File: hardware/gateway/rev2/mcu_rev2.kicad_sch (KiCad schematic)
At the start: 35 parts, among them IC1 STM8L151K4T6, IC5 MB85RC64TAPNF-G-BDERE1, J1 G8250041000YEU, J2 M20-9770342, Q1 IRLML6402TRPBF, U1 2462

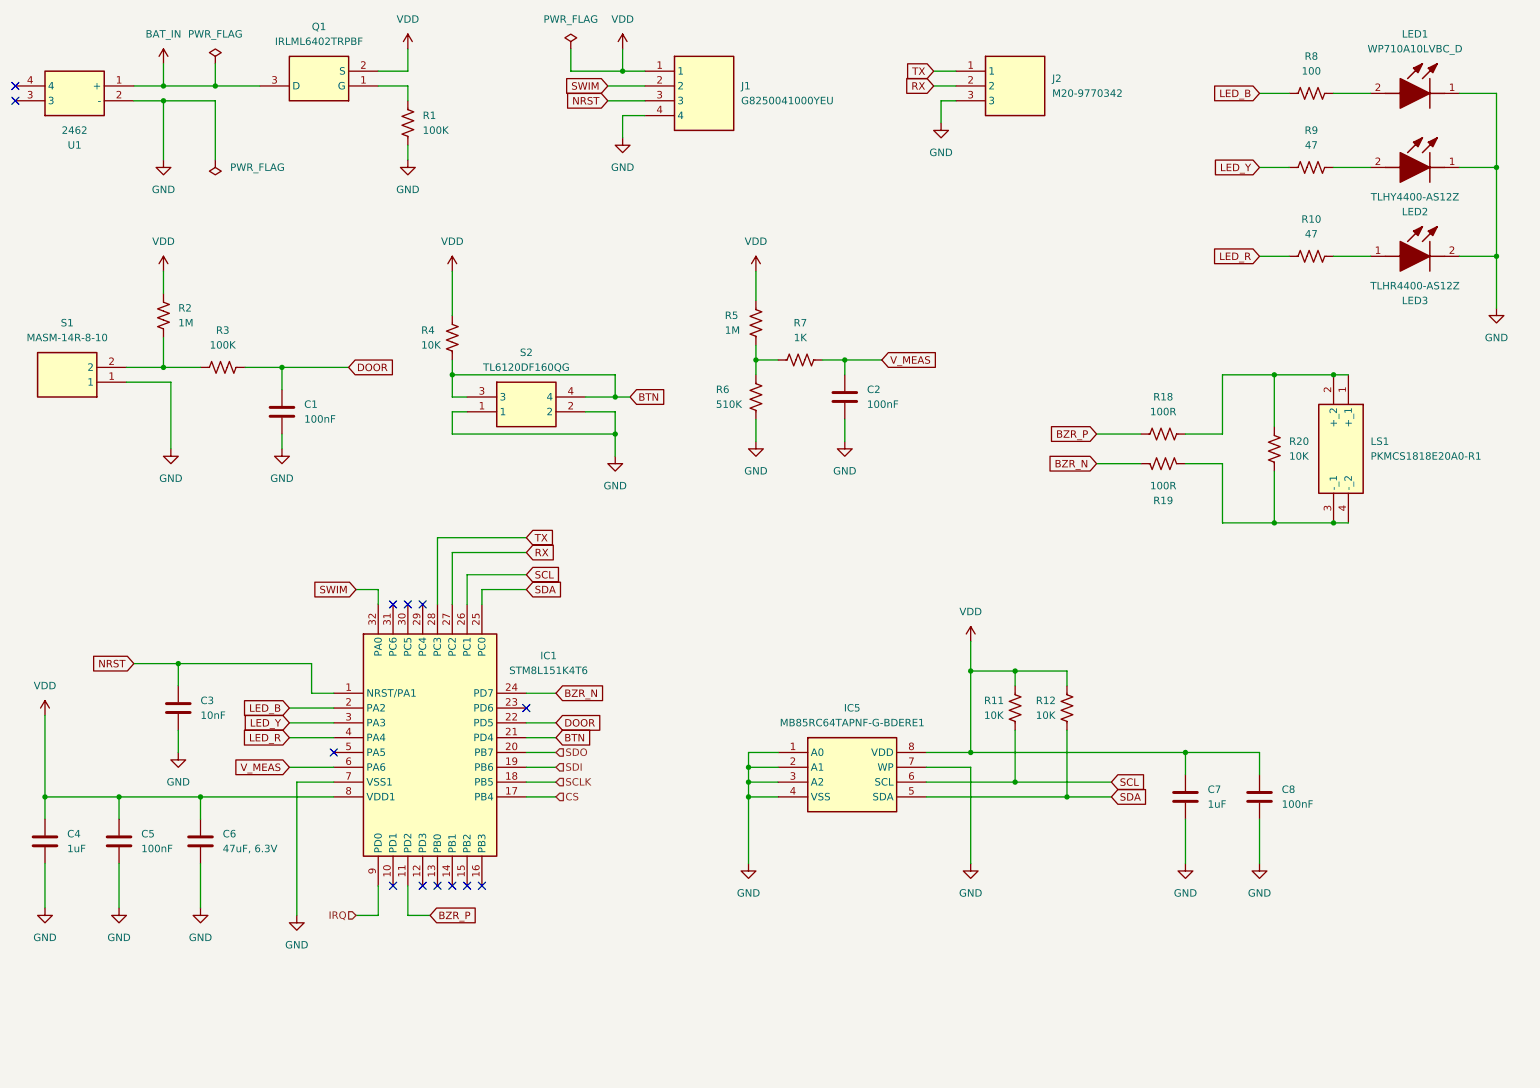
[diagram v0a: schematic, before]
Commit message: EG-59 Schematic with the needed components, plus PCB.
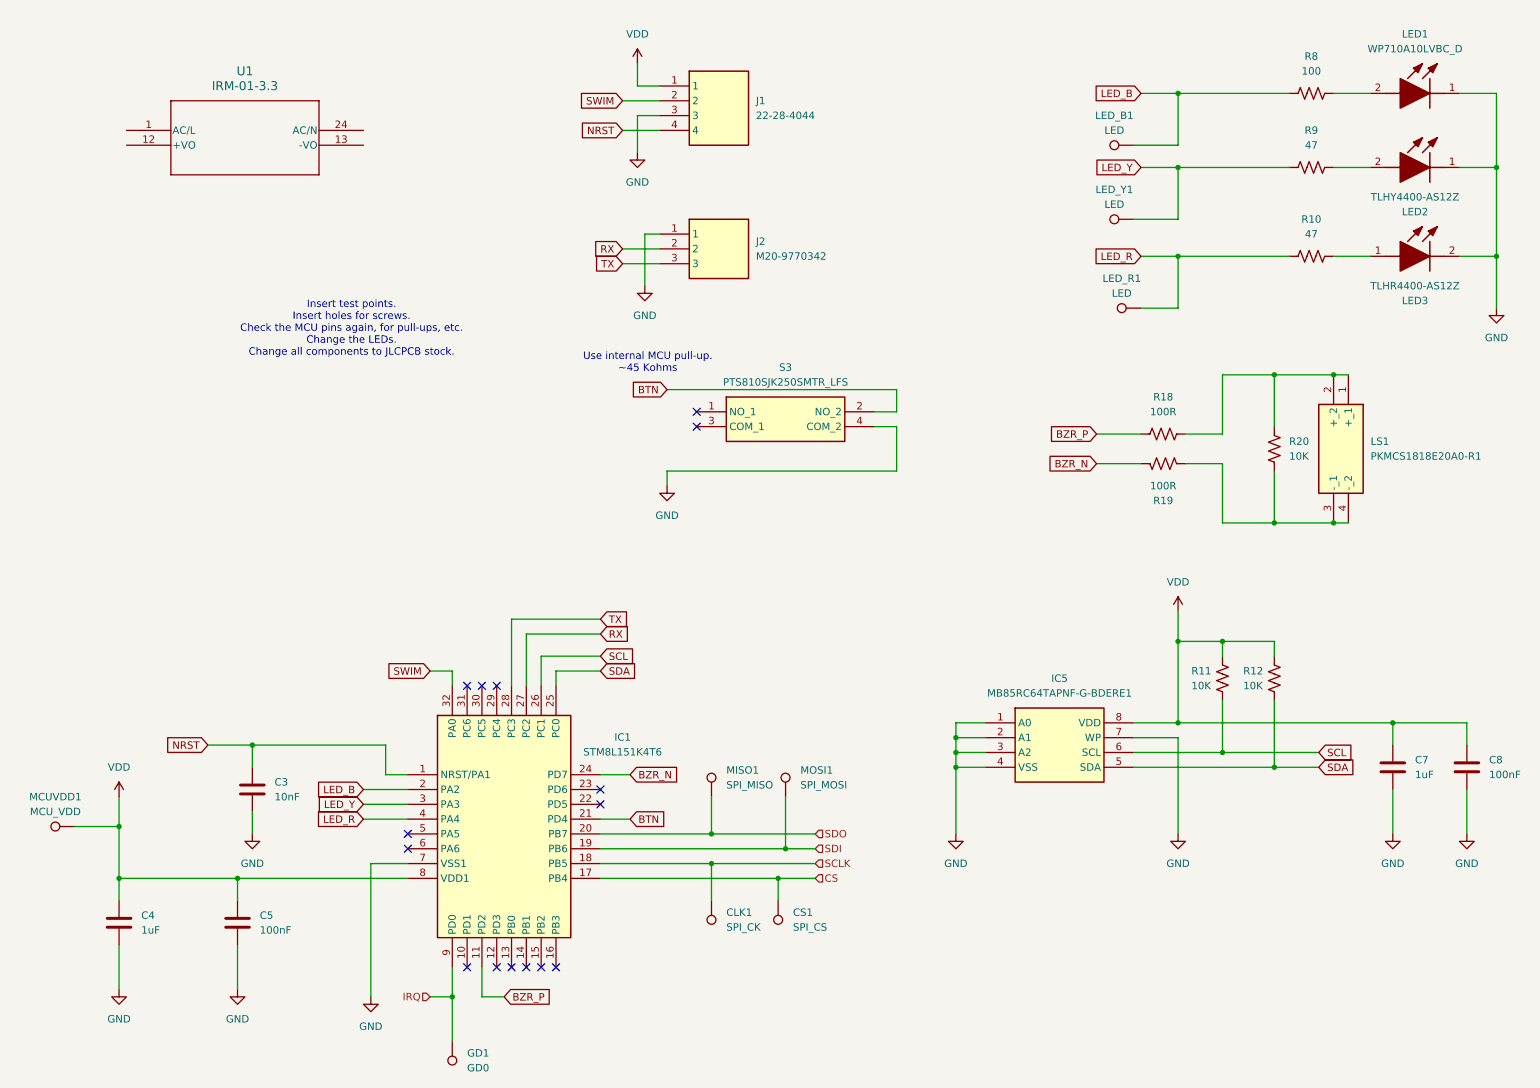
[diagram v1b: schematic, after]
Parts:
- removed C1, C2: 100nF, Capacitor_SMD:C_0603_1608Metric, symbol Device:C
- removed C6: 47uF, 6.3V, Capacitor_SMD:C_1206_3216Metric, symbol Device:C
- removed J1: G8250041000YEU, MyParts:HDRV4W55P0X200_1X4_800X200X635P, symbol G8250041000YEU:G8250041000YEU
- removed Q1: IRLML6402TRPBF, MyParts:SOT95P237X112-3N, symbol IRLML6402TRPBF:IRLML6402TRPBF
- removed R1, R3: 100K, Resistor_SMD:R_0603_1608Metric, symbol Device:R_US
- removed R2, R5: 1M, Resistor_SMD:R_0603_1608Metric, symbol Device:R_US
- removed R4: 10K, Resistor_SMD:R_0603_1608Metric, symbol Device:R_US
- removed R6: 510K, Resistor_SMD:R_0603_1608Metric, symbol Device:R_US
- removed R7: 1K, Resistor_SMD:R_0603_1608Metric, symbol Device:R_US
- removed S1: MASM-14R-8-10, MyParts:MASM14R810, symbol MASM-14R-8-10:MASM-14R-8-10
- removed S2: TL6120DF160QG, MyParts:TL6120DF160QG, symbol TL6120DF160QG:TL6120DF160QG
- removed U1: 2462, MyParts:2462, symbol 2462:2462
- added CLK1: SPI_CK, TestPoint:TestPoint_Pad_D1.0mm, symbol Connector:TestPoint
- added CS1: SPI_CS, TestPoint:TestPoint_Pad_D1.0mm, symbol Connector:TestPoint
- added GD1: GD0, TestPoint:TestPoint_Pad_D1.0mm, symbol Connector:TestPoint
- added J1: 22-28-4044, MyParts:HDRV4W66P0X254_1X4_1016X249X1067P, symbol 22-28-4044:22-28-4044
- added LED_B1, LED_R1, LED_Y1: LED, TestPoint:TestPoint_Pad_D1.0mm, symbol Connector:TestPoint
- added MCUVDD1: MCU_VDD, TestPoint:TestPoint_Pad_D1.0mm, symbol Connector:TestPoint
- added MISO1: SPI_MISO, TestPoint:TestPoint_Pad_D1.0mm, symbol Connector:TestPoint
- added MOSI1: SPI_MOSI, TestPoint:TestPoint_Pad_D1.0mm, symbol Connector:TestPoint
- added S3: PTS810SJK250SMTR_LFS, MyParts:PTS810SJK250SMTRLFS, symbol PTS810SJK250SMTR_LFS:PTS810SJK250SMTR_LFS
- added U1: IRM-01-3.3, MyParts:IRM-01-3-3, symbol IRM-01-3-3:IRM-01-3.3
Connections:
- net BTN: now also S3.2 (NO_2)
- net CS: now also CS1.1
- net GND: now also J2.1, J1.3, S3.4 (COM_2); no longer J2.3
- net IRQ: now also GD1.1
- net LED_B: now also LED_B1.1
- net LED_R: now also LED_R1.1
- net LED_Y: now also LED_Y1.1
- net NRST: now also J1.4
- net SCLK: now also CLK1.1
- net SDI: now also MOSI1.1
- net SDO: now also MISO1.1
- net SWIM: now also J1.2
- net TX: now also J2.3; no longer J2.1
- net VDD: now also J1.1, MCUVDD1.1
- net DOOR: no longer names the net of IC1.22 (PD5)
- net V_MEAS: no longer names the net of IC1.6 (PA6)
- no-connect marks 13 -> 15
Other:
- note added: "Insert test points. Insert holes for screws. Check the MCU pins again, for pull-ups, etc. Change the LEDs. Change all components to JLCPCB stock."
- note added: "Use internal MCU pull-up. ~45 Kohms"
- moved on the sheet: C3, C4, C5, C7, C8, IC1, IC5, J2, R11, R12
